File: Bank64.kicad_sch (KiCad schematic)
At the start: 2 parts, among them U1 XCKU5P-FFVB676

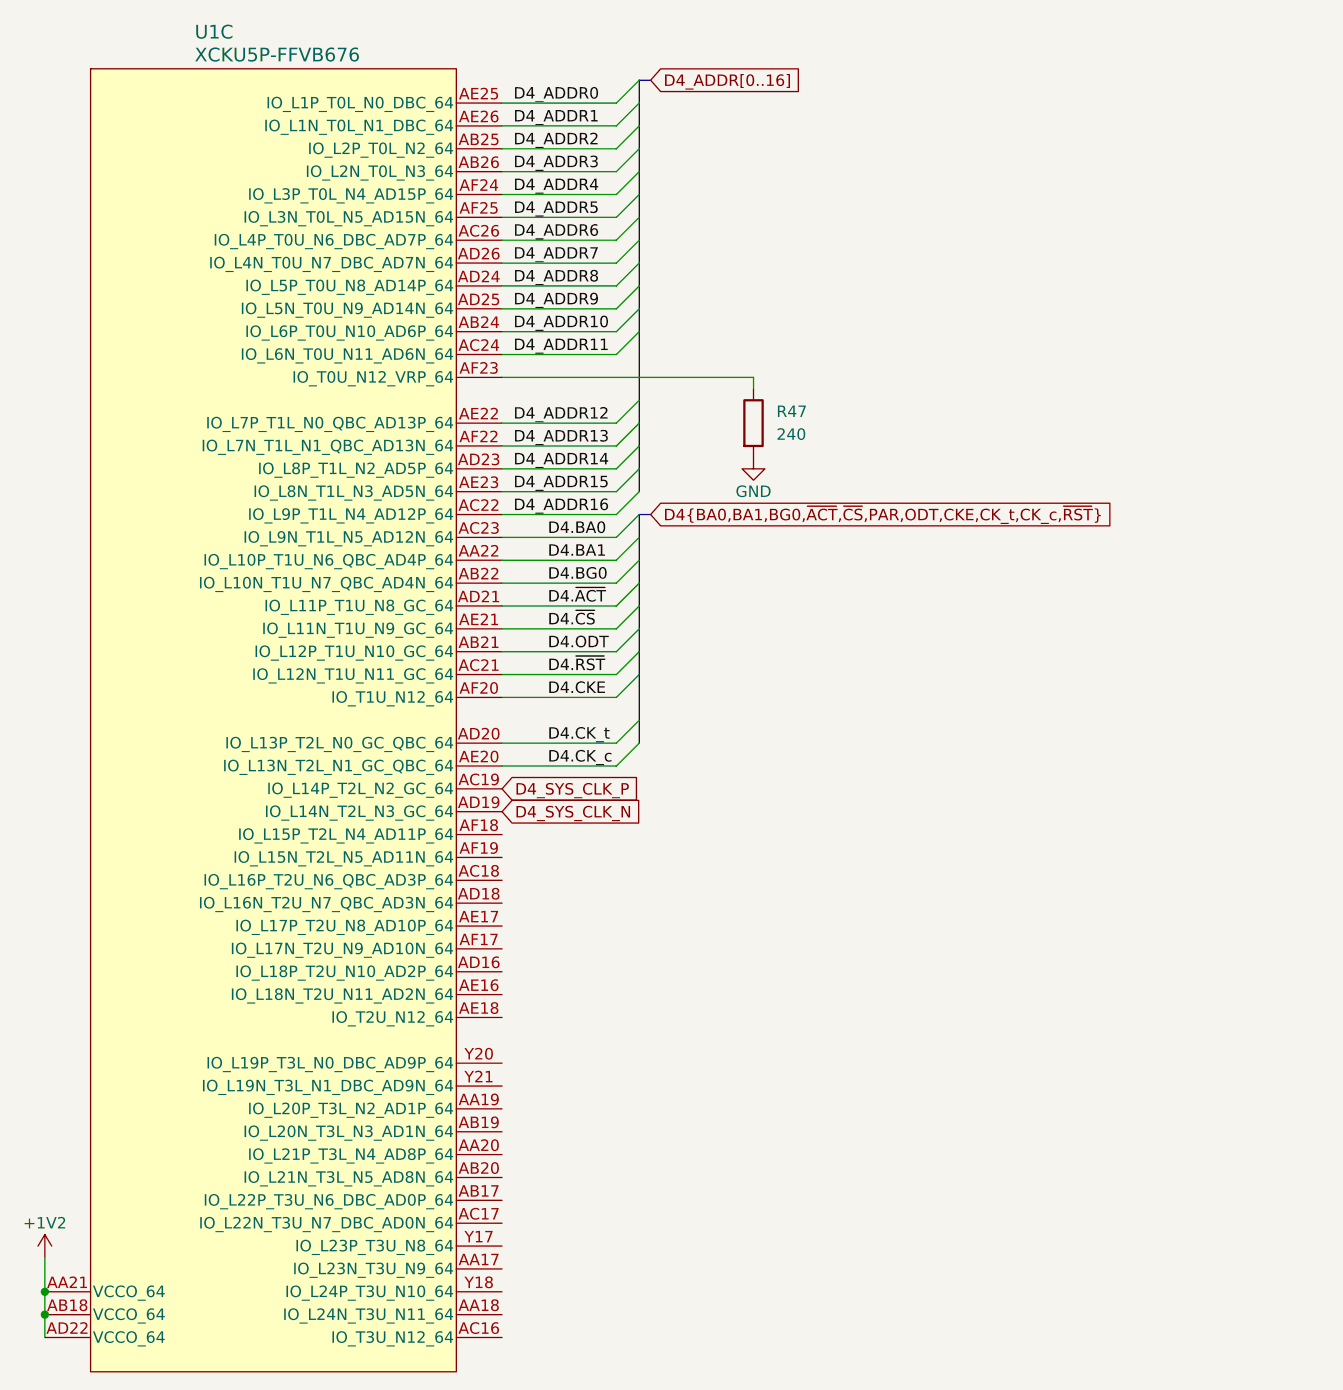
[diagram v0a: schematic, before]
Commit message: finishing schematic
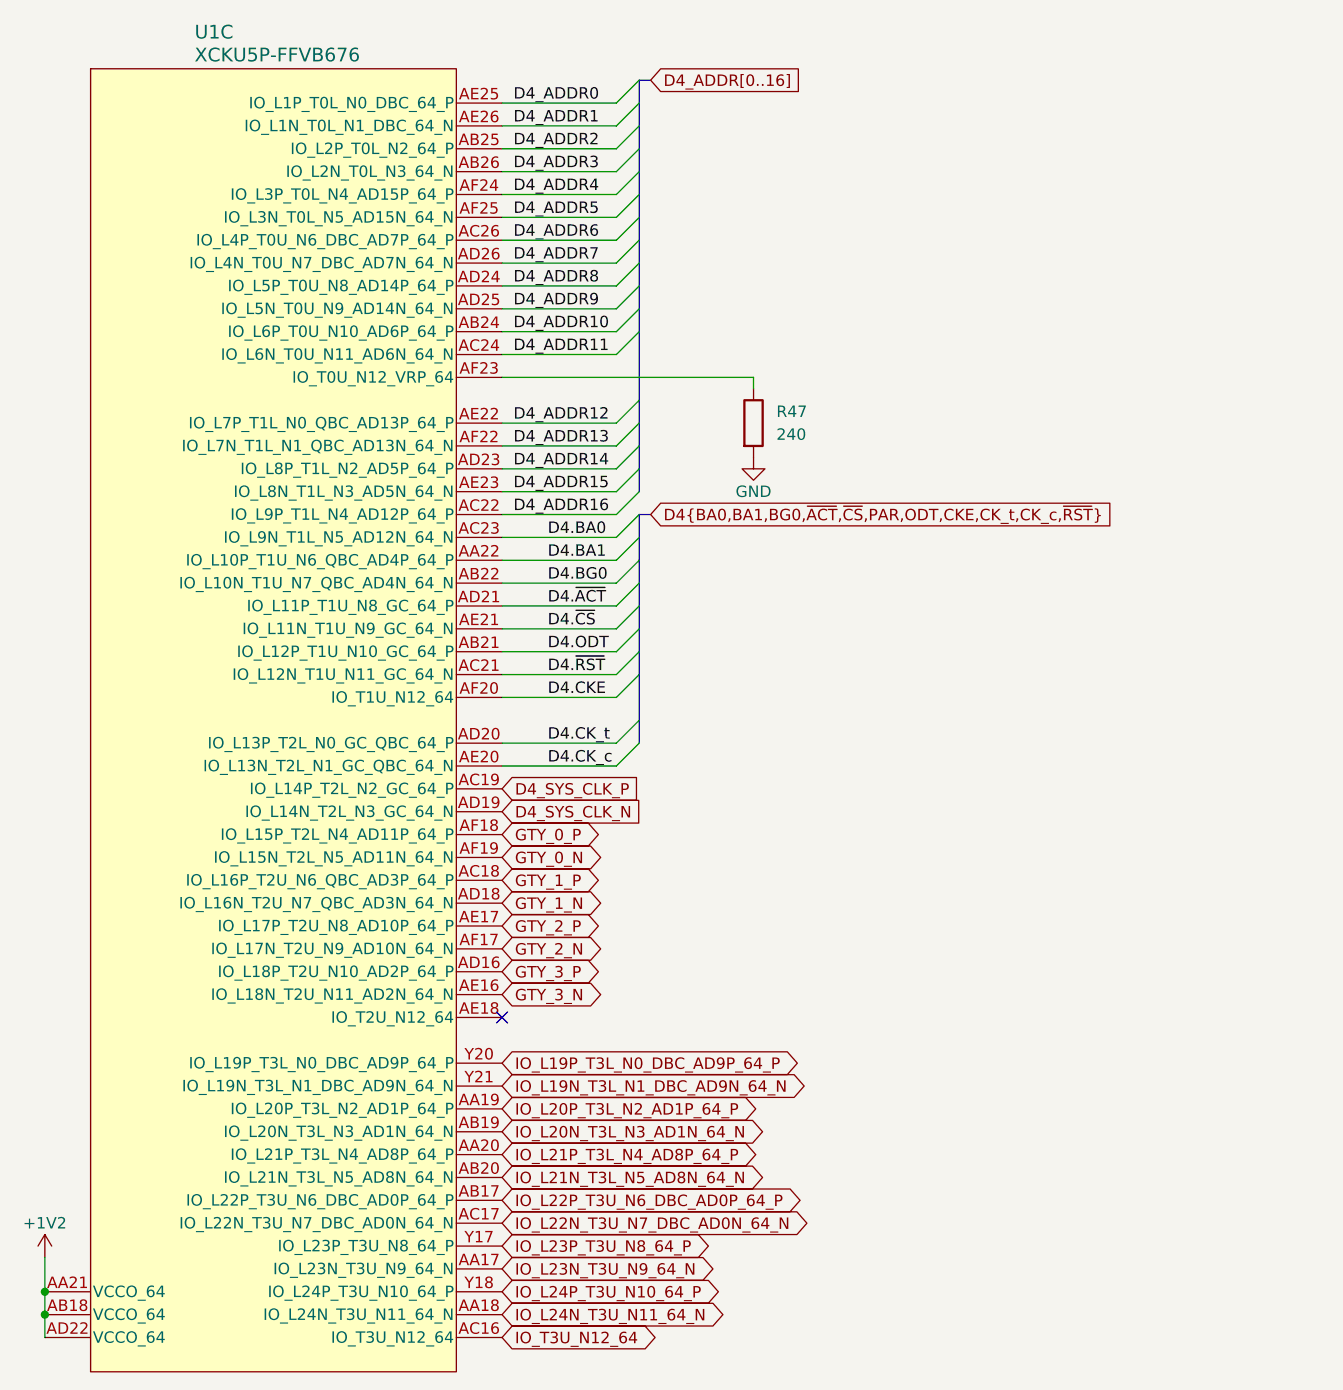
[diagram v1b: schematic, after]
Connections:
- net IO_L23N_T3U_N9_64_N: now reaches U1.AA17 (IO_L23N_T3U_N9_64_N)
- net IO_L24N_T3U_N11_64_N: now reaches U1.AA18 (IO_L24N_T3U_N11_64_N)
- net IO_L20P_T3L_N2_AD1P_64_P: now reaches U1.AA19 (IO_L20P_T3L_N2_AD1P_64_P)
- net IO_L21P_T3L_N4_AD8P_64_P: now reaches U1.AA20 (IO_L21P_T3L_N4_AD8P_64_P)
- net IO_L22P_T3U_N6_DBC_AD0P_64_P: now reaches U1.AB17 (IO_L22P_T3U_N6_DBC_AD0P_64_P)
- net IO_L20N_T3L_N3_AD1N_64_N: now reaches U1.AB19 (IO_L20N_T3L_N3_AD1N_64_N)
- net IO_L21N_T3L_N5_AD8N_64_N: now reaches U1.AB20 (IO_L21N_T3L_N5_AD8N_64_N)
- net IO_T3U_N12_64: now reaches U1.AC16 (IO_T3U_N12_64)
- net IO_L22N_T3U_N7_DBC_AD0N_64_N: now reaches U1.AC17 (IO_L22N_T3U_N7_DBC_AD0N_64_N)
- net GTY_1_P: now reaches U1.AC18 (IO_L16P_T2U_N6_QBC_AD3P_64_P)
- net GTY_3_P: now reaches U1.AD16 (IO_L18P_T2U_N10_AD2P_64_P)
- net GTY_1_N: now reaches U1.AD18 (IO_L16N_T2U_N7_QBC_AD3N_64_N)
- net GTY_3_N: now reaches U1.AE16 (IO_L18N_T2U_N11_AD2N_64_N)
- net GTY_2_P: now reaches U1.AE17 (IO_L17P_T2U_N8_AD10P_64_P)
- net GTY_2_N: now reaches U1.AF17 (IO_L17N_T2U_N9_AD10N_64_N)
- net GTY_0_P: now reaches U1.AF18 (IO_L15P_T2L_N4_AD11P_64_P)
- net GTY_0_N: now reaches U1.AF19 (IO_L15N_T2L_N5_AD11N_64_N)
- net IO_L23P_T3U_N8_64_P: now reaches U1.Y17 (IO_L23P_T3U_N8_64_P)
- net IO_L24P_T3U_N10_64_P: now reaches U1.Y18 (IO_L24P_T3U_N10_64_P)
- net IO_L19P_T3L_N0_DBC_AD9P_64_P: now reaches U1.Y20 (IO_L19P_T3L_N0_DBC_AD9P_64_P)
- net IO_L19N_T3L_N1_DBC_AD9N_64_N: now reaches U1.Y21 (IO_L19N_T3L_N1_DBC_AD9N_64_N)
- no-connect marks 0 -> 1
